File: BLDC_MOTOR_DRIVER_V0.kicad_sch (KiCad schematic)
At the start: 8 parts, among them Q1 N-MOSFET, Q2 N-MOSFET, Q3 N-MOSFET, Q4 N-MOSFET, Q5 N-MOSFET, Q6 N-MOSFET, U1 3-phase Gate Driver, U2 Micro controller

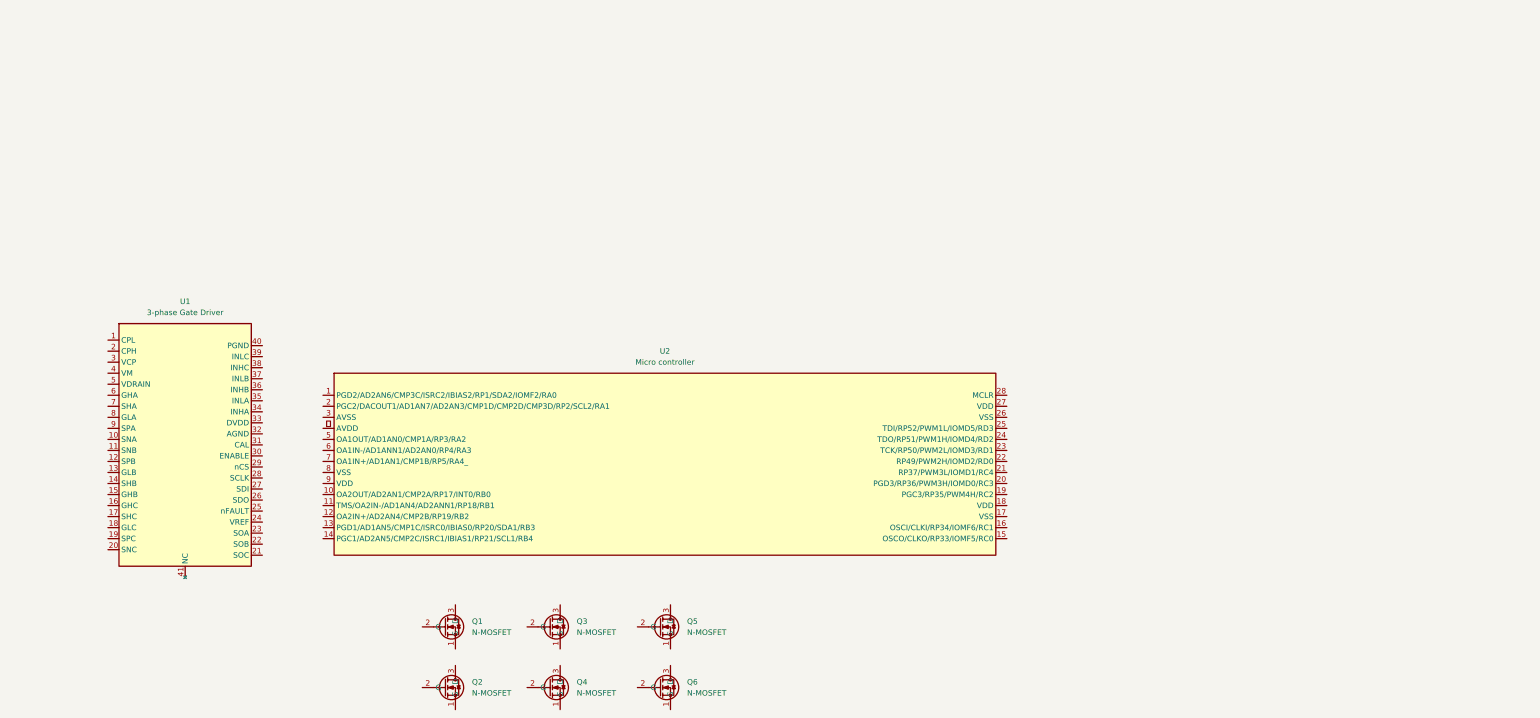
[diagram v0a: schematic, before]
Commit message: update lib
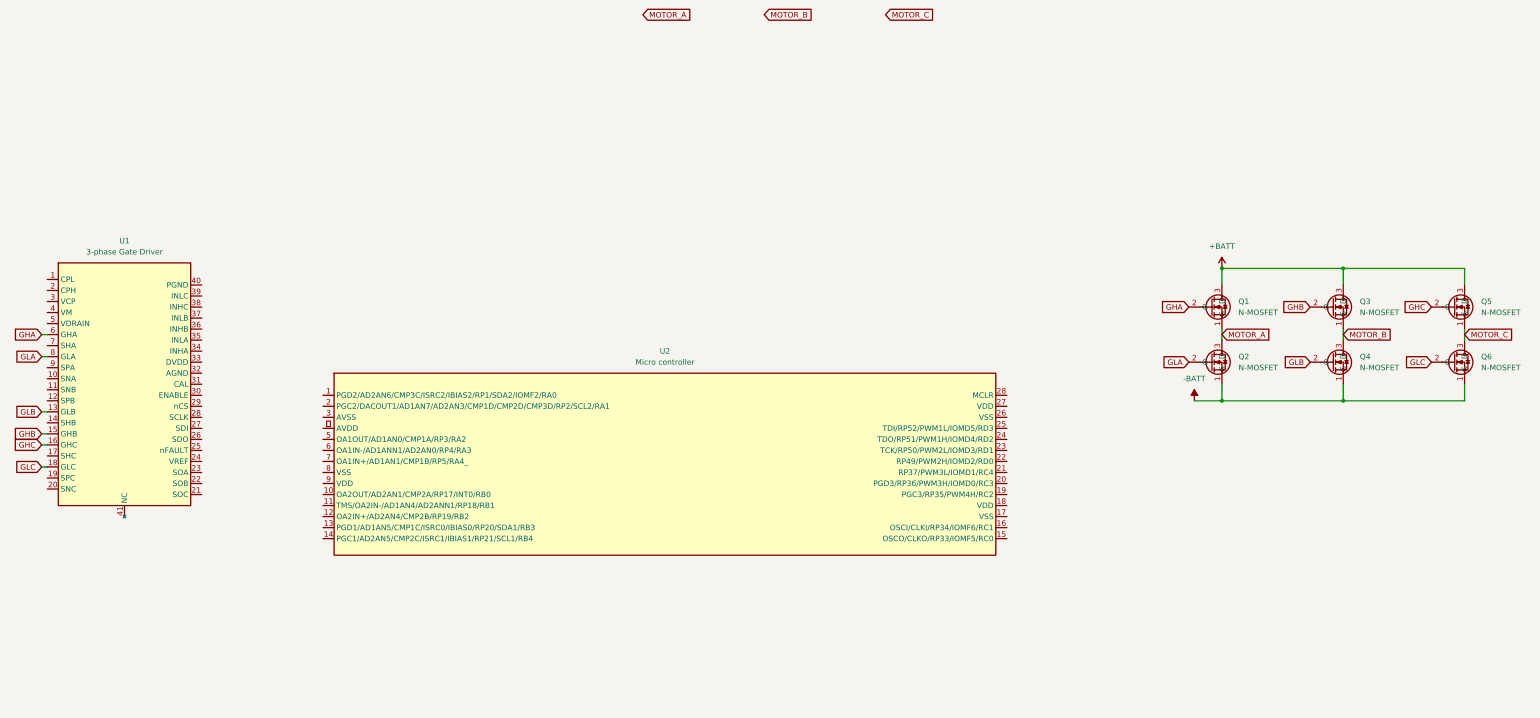
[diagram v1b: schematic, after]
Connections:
- net -BATT: now reaches Q2.1 (S)
- net -BATT: now also Q4.1 (S), Q6.1 (S)
- net GLA: now reaches Q2.2 (G)
- net GLA: now also U1.8 (GLA)
- net MOTOR_A: now reaches Q2.3 (D)
- net MOTOR_A: now also Q1.1 (S)
- net MOTOR_C: now reaches Q5.1 (S)
- net MOTOR_C: now also Q6.3 (D)
- net GHC: now reaches Q5.2 (G)
- net GHC: now also U1.16 (GHC)
- net +BATT: now reaches Q5.3 (D)
- net +BATT: now also Q1.3 (D), Q3.3 (D)
- net GHA: now reaches Q1.2 (G)
- net GHA: now also U1.6 (GHA)
- net GLB: now reaches Q4.2 (G)
- net GLB: now also U1.13 (GLB)
- net MOTOR_B: now reaches Q4.3 (D)
- net MOTOR_B: now also Q3.1 (S)
- net GLC: now reaches Q6.2 (G)
- net GLC: now also U1.18 (GLC)
- net GHB: now reaches Q3.2 (G)
- net GHB: now also U1.15 (GHB)
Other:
- moved on the sheet: Q1, Q2, Q3, Q4, Q5, Q6, U1
